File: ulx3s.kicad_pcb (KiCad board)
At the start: 4 copper layers, 94 x 50.8 mm, 119 parts, among them J1 CONN_02X20, J2 CONN_02X20, J3 WIFI_OFF, J4 CONN_02X03, Q1 BC857, Q2 2N7002, U10 S25FL164K0XMFI011, U11 PCA9306DCTR, U2 ESP-32S, U3 AP3429A, U4 AP3429A, U5 AP3429A, U6 FT231XS, U7 PCF8523, U8 MAX11123, U9 MT48LC4M16A2TG, Y1 FNETHE025

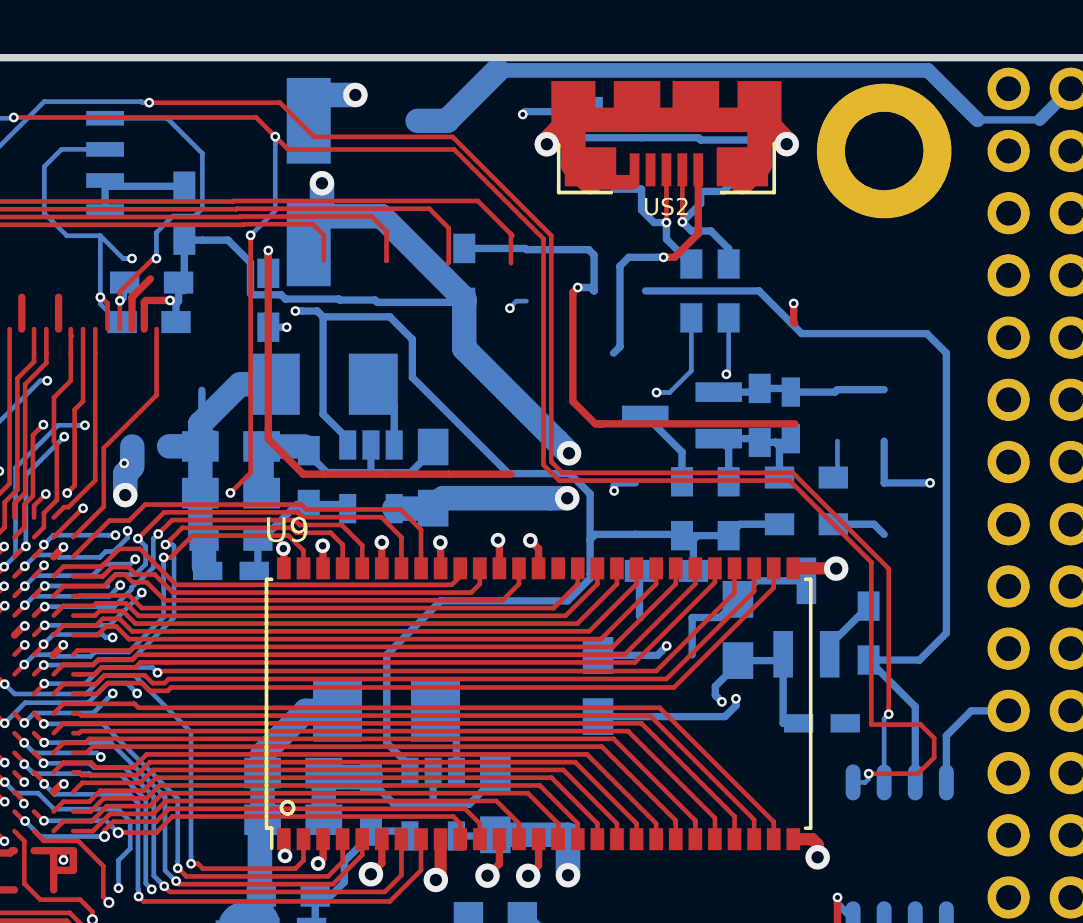
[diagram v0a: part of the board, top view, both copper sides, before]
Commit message: small track cosmetics
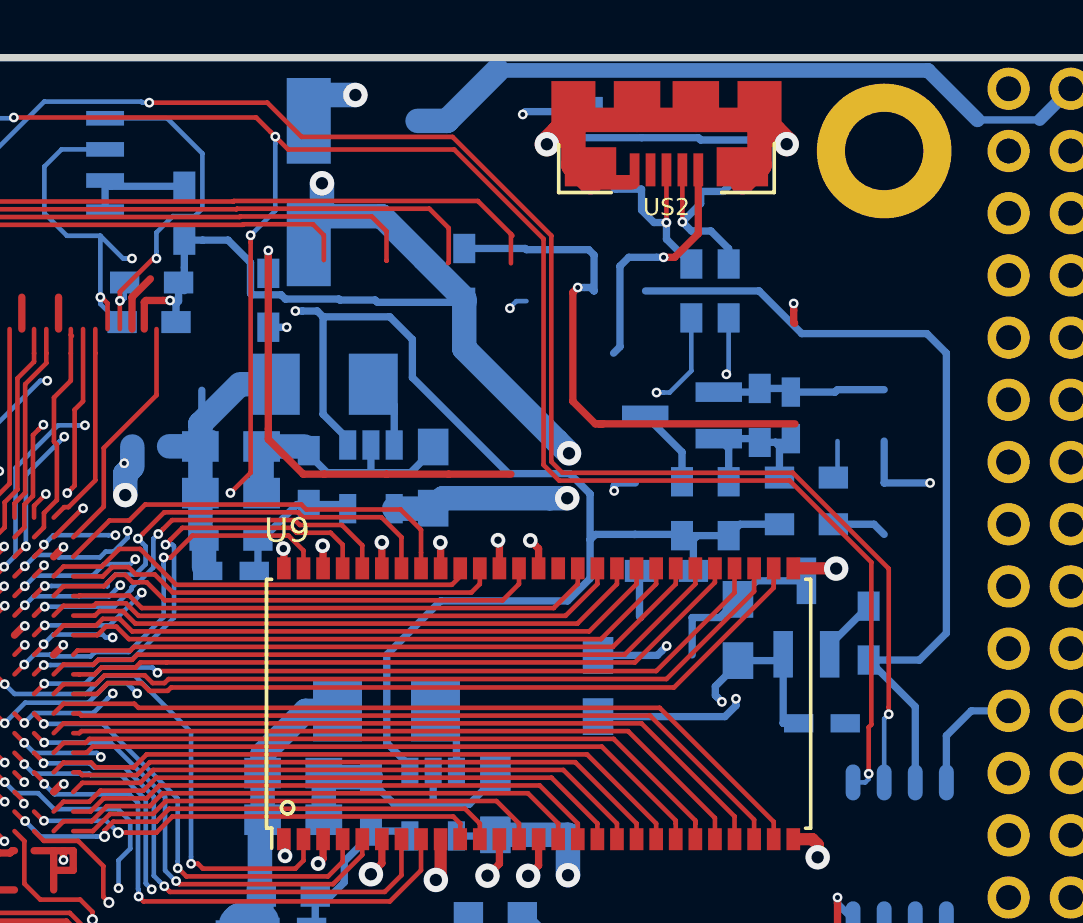
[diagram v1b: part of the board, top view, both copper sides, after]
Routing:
- net GPDI_SDA: track 89.4 -> 84.9 mm
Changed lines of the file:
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@@
     (thickness 1.6)
     (drawings 28)
-    (tracks 4125)
+    (tracks 4121)
     (zones 0)
     (modules 160)
@@
   (via (at 134.48 91) (size 0.4) (drill 0.2) (layers F.Cu B.Cu) (net 14))
   (segment (start 134.88 90.6) (end 134.48 91) (width 0.3) (layer F.Cu) (net 14))
+  (segment (start 167.18355 81.105) (end 167.18355 82.68145) (width 0.3) (layer B.Cu) (net 15))
+  (segment (start 166.265 83.6) (end 161.08 83.6) (width 0.3) (layer B.Cu) (net 15))
+  (segment (start 167.18355 82.68145) (end 166.265 83.6) (width 0.3) (layer B.Cu) (net 15))
+  (segment (start 161.08 83.6) (end 158.88 85.8) (width 0.3) (layer B.Cu) (net 15))
+  (segment (start 158.88 85.8) (end 158.88 89.4) (width 0.3) (layer B.Cu) (net 15))
+  (segment (start 158.88 89.4) (end 159.825 90.345) (width 0.3) (layer B.Cu) (net 15))
+  (segment (start 159.825 90.345) (end 159.825 90.6) (width 0.3) (layer B.Cu) (net 15))
   (segment (start 121.086654 69.078528) (end 121.086654 70.584047) (width 0.3) (layer In1.Cu) (net 15))
   (segment (start 121.086654 69.078528) (end 121.1508 69.142674) (width 0.3) (layer In2.Cu) (net 15))
@@
   (segment (start 156.044535 71.764535) (end 155.432202 71.764535) (width 0.3) (layer B.Cu) (net 15))
   (segment (start 155.432202 71.764535) (end 155.14936 71.764535) (width 0.3) (layer B.Cu) (net 15))
-  (segment (start 167.18355 81.105) (end 167.18355 82.51855) (width 0.3) (layer B.Cu) (net 15))
   (segment (start 169.03 80.885) (end 167.40355 80.885) (width 0.3) (layer B.Cu) (net 15))
   (segment (start 167.40355 80.885) (end 167.18355 81.105) (width 0.3) (layer B.Cu) (net 15))
-  (segment (start 166.265 83.6) (end 167.265 82.6) (width 0.3) (layer B.Cu) (net 15))
-  (segment (start 167.18355 82.51855) (end 167.265 82.6) (width 0.3) (layer B.Cu) (net 15))
   (segment (start 156.28 75.98) (end 156.28 72) (width 0.3) (layer B.Cu) (net 15))
   (segment (start 157.285 77.235) (end 157.285 76.985) (width 0.3) (layer B.Cu) (net 15))
   (segment (start 157.285 76.985) (end 156.28 75.98) (width 0.3) (layer B.Cu) (net 15))
-  (segment (start 159.825 90.6) (end 159.825 90.345) (width 0.3) (layer B.Cu) (net 15))
-  (segment (start 159.825 90.345) (end 158.88 89.4) (width 0.3) (layer B.Cu) (net 15))
-  (segment (start 158.88 89.4) (end 158.88 85.8) (width 0.3) (layer B.Cu) (net 15))
-  (segment (start 158.88 85.8) (end 161.08 83.6) (width 0.3) (layer B.Cu) (net 15))
-  (segment (start 161.08 83.6) (end 166.265 83.6) (width 0.3) (layer B.Cu) (net 15))
   (segment (start 168.98 80.885) (end 169.03 80.885) (width 0.3) (layer B.Cu) (net 15))
   (segment (start 169.03 80.885) (end 170.885 80.885) (width 0.3) (layer B.Cu) (net 15))
@@
   (via (at 147.983153 71.34708) (size 0.4) (drill 0.2) (layers F.Cu B.Cu) (net 37))
   (via (at 149.475951 69.619684) (size 0.4) (drill 0.2) (layers F.Cu B.Cu) (net 37))
+  (segment (start 178.665908 88.648967) (end 178.55819 88.756685) (width 0.19) (layer F.Cu) (net 38))
+  (segment (start 178.55819 88.756685) (end 178.55819 90.656032) (width 0.19) (layer F.Cu) (net 38))
   (segment (start 165.918477 78.686028) (end 175.33012 78.686028) (width 0.19) (layer F.Cu) (net 38))
   (segment (start 161.633939 65.170215) (end 165.282602 68.818878) (width 0.19) (layer F.Cu) (net 38))
   (segment (start 177.92 91.011) (end 178.4148 91.011) (width 0.19) (layer B.Cu) (net 38))
-  (segment (start 181.231033 89.20607) (end 181.231033 89.99393) (width 0.19) (layer F.Cu) (net 38))
   (via (at 178.55819 90.656032) (size 0.4) (drill 0.2) (layers F.Cu B.Cu) (net 38))
   (segment (start 178.55819 90.86761) (end 178.55819 90.656032) (width 0.19) (layer B.Cu) (net 38))
-  (segment (start 178.665908 88.648967) (end 180.67393 88.648967) (width 0.19) (layer F.Cu) (net 38))
   (segment (start 178.4148 91.011) (end 178.55819 90.86761) (width 0.19) (layer B.Cu) (net 38))
   (segment (start 154.855774 65.170215) (end 161.633939 65.170215) (width 0.19) (layer F.Cu) (net 38))
   (segment (start 175.33012 78.686028) (end 178.665908 82.021816) (width 0.19) (layer F.Cu) (net 38))
   (segment (start 178.665908 82.021816) (end 178.665908 88.648967) (width 0.19) (layer F.Cu) (net 38))
-  (segment (start 180.67393 88.648967) (end 181.231033 89.20607) (width 0.19) (layer F.Cu) (net 38))
-  (segment (start 181.231033 89.99393) (end 180.568931 90.656032) (width 0.19) (layer F.Cu) (net 38))
   (segment (start 154.329326 64.643767) (end 154.855774 65.170215) (width 0.19) (layer F.Cu) (net 38))
   (segment (start 165.282602 68.818878) (end 165.282602 78.050153) (width 0.19) (layer F.Cu) (net 38))
-  (segment (start 180.568931 90.656032) (end 178.55819 90.656032) (width 0.19) (layer F.Cu) (net 38))
   (segment (start 165.282602 78.050153) (end 165.918477 78.686028) (width 0.19) (layer F.Cu) (net 38))
   (segment (start 148.2539 80.000797) (end 148.254705 79.999992) (width 0.19) (layer In2.Cu) (net 38))
@@
   (segment (start 141.98 63.895) (end 140.055 63.895) (width 0.19) (layer B.Cu) (net 38))
   (segment (start 140.055 63.895) (end 139.82 64.13) (width 0.19) (layer B.Cu) (net 38))
-  (segment (start 179.19 91.011) (end 179.19 88.412934) (width 0.19) (layer B.Cu) (net 39))
-  (via (at 179.375977 88.226957) (size 0.4) (drill 0.2) (layers F.Cu B.Cu) (net 39))
+  (segment (start 149.183754 63.257114) (end 154.004817 63.257114) (width 0.19) (layer F.Cu) (net 39))
   (segment (start 165.599613 77.918843) (end 166.049787 78.369017) (width 0.19) (layer F.Cu) (net 39))
-  (segment (start 179.19 88.412934) (end 179.375977 88.226957) (width 0.19) (layer B.Cu) (net 39))
-  (segment (start 154.520337 63.257114) (end 155.918329 64.655106) (width 0.19) (layer F.Cu) (net 39))
-  (segment (start 161.567151 64.655106) (end 165.599613 68.687568) (width 0.19) (layer F.Cu) (net 39))
+  (segment (start 154.004817 63.257114) (end 155.402809 64.655106) (width 0.19) (layer F.Cu) (net 39))
   (segment (start 175.46143 78.369017) (end 179.375977 82.283564) (width 0.19) (layer F.Cu) (net 39))
-  (segment (start 179.375977 82.283564) (end 179.375977 87.944115) (width 0.19) (layer F.Cu) (net 39))
   (segment (start 179.375977 87.944115) (end 179.375977 88.226957) (width 0.19) (layer F.Cu) (net 39))
-  (segment (start 166.049787 78.369017) (end 175.46143 78.369017) (width 0.19) (layer F.Cu) (net 39))
-  (segment (start 155.918329 64.655106) (end 161.567151 64.655106) (width 0.19) (layer F.Cu) (net 39))
+  (segment (start 155.402809 64.655106) (end 161.567151 64.655106) (width 0.19) (layer F.Cu) (net 39))
+  (segment (start 161.567151 64.655106) (end 165.599613 68.687568) (width 0.19) (layer F.Cu) (net 39))
   (segment (start 165.599613 68.687568) (end 165.599613 77.918843) (width 0.19) (layer F.Cu) (net 39))
-  (segment (start 149.183754 63.257114) (end 154.520337 63.257114) (width 0.19) (layer F.Cu) (net 39))
+  (segment (start 166.049787 78.369017) (end 175.46143 78.369017) (width 0.19) (layer F.Cu) (net 39))
+  (segment (start 179.375977 82.283564) (end 179.375977 87.944115) (width 0.19) (layer F.Cu) (net 39))
+  (segment (start 179.19 91.011) (end 179.19 88.412934) (width 0.19) (layer B.Cu) (net 39))
+  (via (at 179.375977 88.226957) (size 0.4) (drill 0.2) (layers F.Cu B.Cu) (net 39))
+  (segment (start 179.19 88.412934) (end 179.375977 88.226957) (width 0.19) (layer B.Cu) (net 39))
   (segment (start 138.98 68.578574) (end 138.98 67.516) (width 0.19) (layer B.Cu) (net 39))
   (segment (start 140.035989 81.4) (end 140.035989 69.634563) (width 0.19) (layer B.Cu) (net 39))
